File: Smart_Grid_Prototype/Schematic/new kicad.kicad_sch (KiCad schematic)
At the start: 78 parts, among them J1 EXT_POW, J2 AC_LOAD, J3 AC_STEPDOWN, J4 DC_LOAD, J5 POW_SHARE, J6 USB_C_Receptacle_PowerOnly_6P, J7 220VAC, J8 220VAC-TRANS, K1 G3MB-202PDC5, Q1 BD139, Q2 BD139, Q3 BD139, Q4 BD139, Q5 BD139, Q6 BD139, Q7 BD139, Q8 BD139, U1 ESP8266, U10 PC817, U11 PC817, U12 PC817, U13 PC817, U14 PC817, U15 PC817, U16 PC817, U2 RELAY_INT, U3 RELAY_PS, U4 PC817, U5 LM7824_TO220, U6 PC817, U7 PC817, U8 LM317_TO-220, U9 PC817

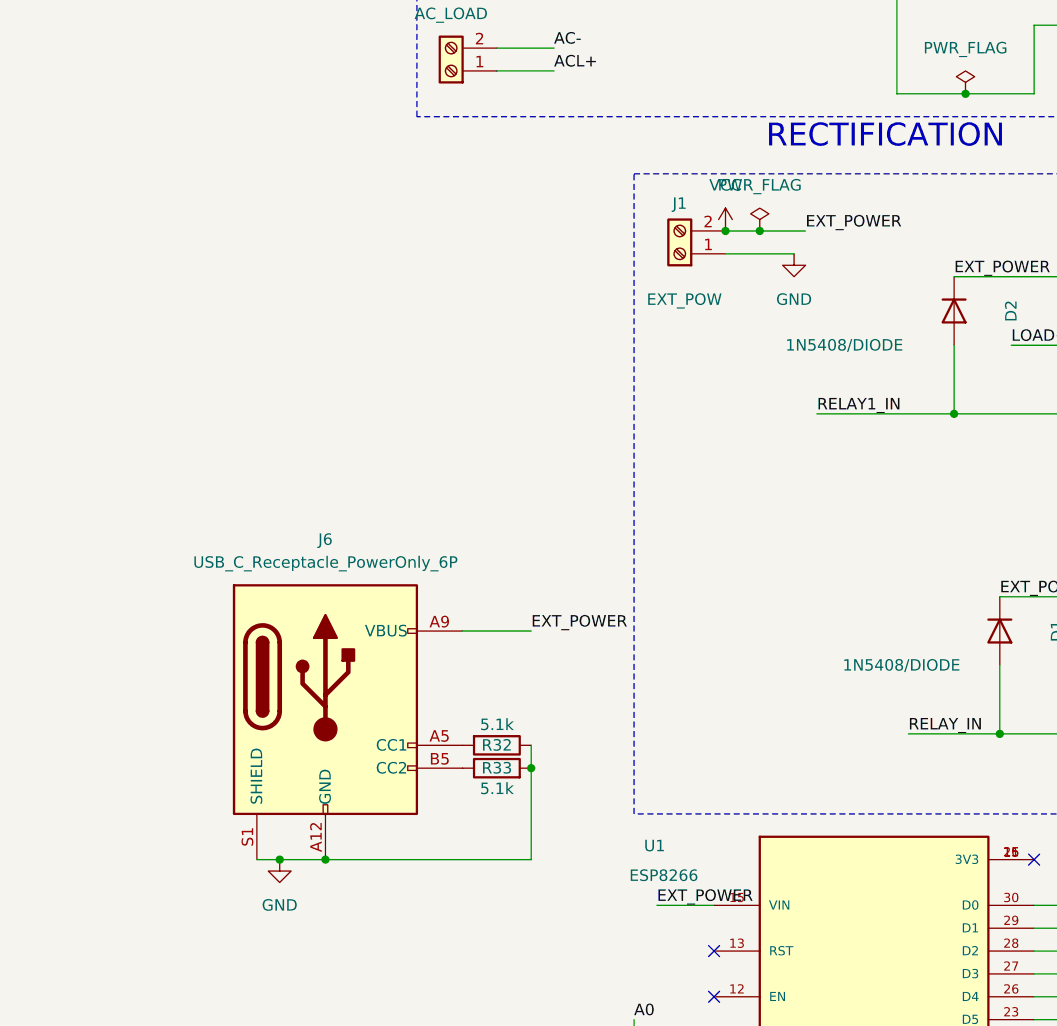
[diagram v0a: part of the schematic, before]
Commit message: finalised
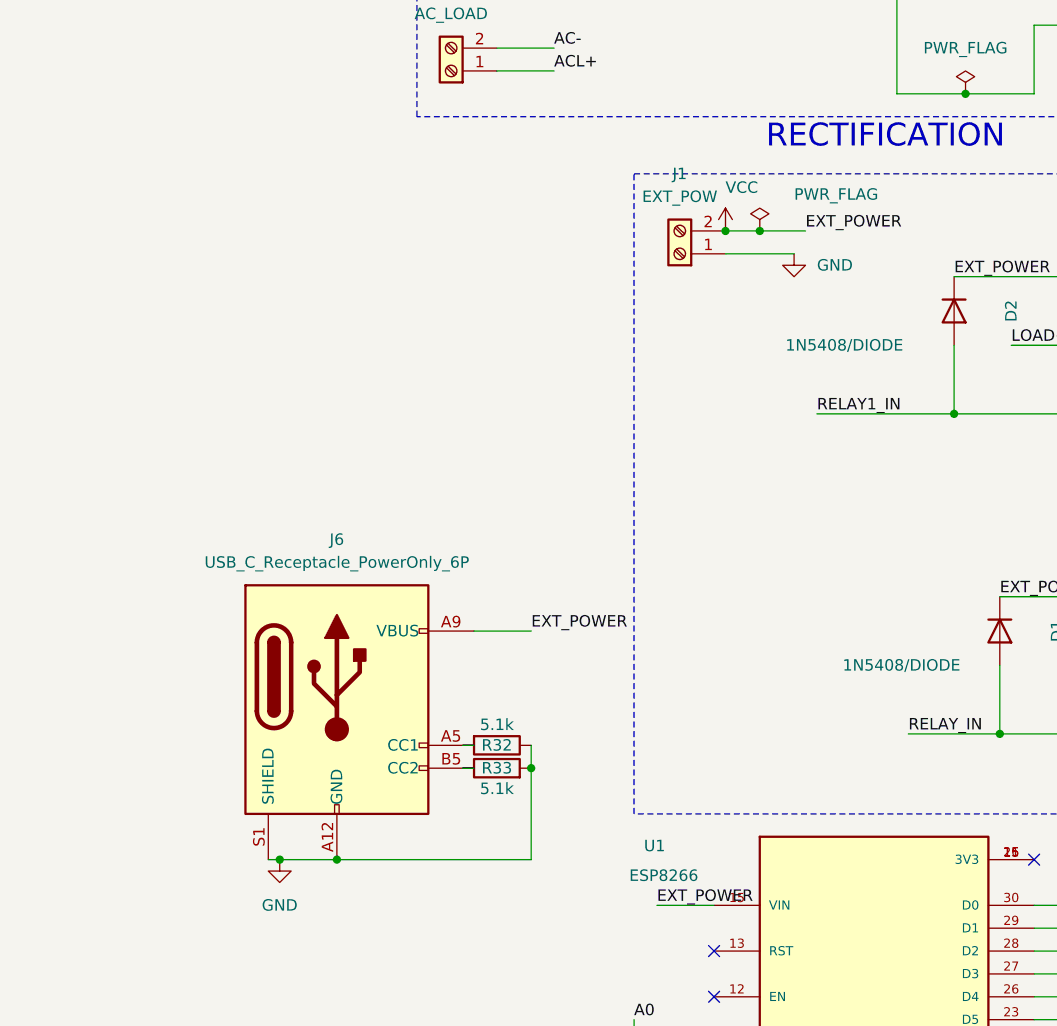
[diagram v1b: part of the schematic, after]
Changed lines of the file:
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@@
 	)
 	(junction
+		(at 69.85 166.37)
+		(diameter 0)
+		(color 0 0 0 0)
+	)
+	(junction
 		(at 139.7 81.28)
 		(diameter 0)
@@
 	)
 	(junction
-		(at 68.58 166.37)
-		(diameter 0)
-		(color 0 0 0 0)
-	)
-	(junction
 		(at 328.93 76.2)
 		(diameter 0)
@@
 	(wire
 		(pts
+			(xy 85.09 153.67) (xy 83.82 153.67)
+		)
+		(stroke
+			(width 0)
+			(type default)
+		)
+	)
+	(wire
+		(pts
 			(xy 323.85 68.58) (xy 323.85 77.47)
 		)
@@
 	(wire
 		(pts
+			(xy 85.09 156.21) (xy 83.82 156.21)
+		)
+		(stroke
+			(width 0)
+			(type default)
+		)
+	)
+	(wire
+		(pts
 			(xy 231.14 210.82) (xy 231.14 209.55)
 		)
@@
 	(wire
 		(pts
-			(xy 63.5 166.37) (xy 68.58 166.37)
-		)
-		(stroke
-			(width 0)
-			(type default)
-		)
-	)
-	(wire
-		(pts
 			(xy 294.64 72.39) (xy 284.48 72.39)
 		)
@@
 	(wire
 		(pts
+			(xy 69.85 166.37) (xy 91.44 166.37)
+		)
+		(stroke
+			(width 0)
+			(type default)
+		)
+	)
+	(wire
+		(pts
 			(xy 356.87 100.33) (xy 361.95 100.33)
 		)
@@
 	(wire
 		(pts
-			(xy 83.82 140.97) (xy 91.44 140.97)
+			(xy 85.09 140.97) (xy 91.44 140.97)
 		)
 		(stroke
@@
 	(wire
 		(pts
-			(xy 60.96 166.37) (xy 63.5 166.37)
+			(xy 62.23 166.37) (xy 63.5 166.37)
 		)
 		(stroke
@@
 	(wire
 		(pts
-			(xy 91.44 166.37) (xy 68.58 166.37)
+			(xy 63.5 166.37) (xy 69.85 166.37)
 		)
 		(stroke
@@
 		)
 		(property "Value" "GND"
-			(at 120.65 104.14 0)
+			(at 123.19 100.3299 0)
 			(effects
 				(font
 					(size 1.27 1.27)
 				)
+				(justify left)
 			)
 		)
@@
 		(on_board yes)
 		(dnp no)
-		(fields_autoplaced yes)
 		(property "Reference" "#PWR017"
 			(at 113.03 100.33 0)
@@
 		)
 		(property "Value" "VCC"
-			(at 113.03 91.44 0)
+			(at 113.03 91.694 0)
 			(effects
 				(font
 					(size 1.27 1.27)
 				)
+				(justify left)
 			)
 		)
@@
 		(on_board yes)
 		(dnp no)
-		(fields_autoplaced yes)
 		(property "Reference" "#FLG04"
 			(at 116.84 94.615 0)
@@
 		)
 		(property "Value" "PWR_FLAG"
-			(at 116.84 91.44 0)
+			(at 120.65 92.456 0)
 			(effects
 				(font
 					(size 1.27 1.27)
 				)
+				(justify left)
 			)
 		)
@@
 	)
 	(symbol
-		(lib_id "Connector:USB_C_Receptacle_PowerOnly_6P")
-		(at 68.58 148.59 0)
-		(unit 1)
-		(exclude_from_sim no)
-		(in_bom yes)
-		(on_board yes)
-		(dnp no)
-		(fields_autoplaced yes)
-		(property "Reference" "J6"
-			(at 68.58 130.81 0)
-			(effects
-				(font
-					(size 1.27 1.27)
-				)
-			)
-		)
-		(property "Value" "USB_C_Receptacle_PowerOnly_6P"
-			(at 68.58 133.35 0)
-			(effects
-				(font
-					(size 1.27 1.27)
-				)
-			)
-		)
-		(property "Footprint" "Connector_USB:USB_C_Receptacle_GCT_USB4125-xx-x-0190_6P_TopMnt_Horizontal"
-			(at 72.39 146.05 0)
-			(effects
-				(font
-					(size 1.27 1.27)
-				)
-				(hide yes)
-			)
-		)
-		(property "Datasheet" "https://www.usb.org/sites/default/files/documents/usb_type-c.zip"
-			(at 68.58 148.59 0)
-			(effects
-				(font
-					(size 1.27 1.27)
-				)
-				(hide yes)
-			)
-		)
-		(property "Description" "USB Power-Only 6P Type-C Receptacle connector"
-			(at 68.58 148.59 0)
-			(effects
-				(font
-					(size 1.27 1.27)
-				)
-				(hide yes)
-			)
-		)
-		(pin "S1"
-		)
-		(pin "B12"
-		)
-		(pin "B9"
-		)
-		(pin "B5"
-		)
-		(pin "A12"
-		)
-		(pin "A5"
-		)
-		(pin "A9"
-		)
-		(instances
-			(project ""
-				(path "/e03aa56c-38cd-4df1-a477-6f5e62efd874"
-					(reference "J6")
-					(unit 1)
-				)
-			)
-		)
-	)
-	(symbol
 		(lib_id "Device:R")
 		(at 53.34 49.53 270)
@@
 	)
 	(symbol
+		(lib_id "Connector:USB_C_Receptacle_PowerOnly_6P")
+		(at 69.85 148.59 0)
+		(unit 1)
+		(exclude_from_sim no)
+		(in_bom yes)
+		(on_board yes)
+		(dnp no)
+		(fields_autoplaced yes)
+		(property "Reference" "J6"
+			(at 69.85 130.81 0)
+			(effects
+				(font
+					(size 1.27 1.27)
+				)
+			)
+		)
+		(property "Value" "USB_C_Receptacle_PowerOnly_6P"
+			(at 69.85 133.35 0)
+			(effects
+				(font
+					(size 1.27 1.27)
+				)
+			)
+		)
+		(property "Footprint" "Connector_USB:USB_C_Receptacle_GCT_USB4125-xx-x-0190_6P_TopMnt_Horizontal"
+			(at 73.66 146.05 0)
+			(effects
+				(font
+					(size 1.27 1.27)
+				)
+				(hide yes)
+			)
+		)
+		(property "Datasheet" "https://www.usb.org/sites/default/files/documents/usb_type-c.zip"
+			(at 69.85 148.59 0)
+			(effects
+				(font
+					(size 1.27 1.27)
+				)
+				(hide yes)
+			)
+		)
+		(property "Description" "USB Power-Only 6P Type-C Receptacle connector"
+			(at 69.85 148.59 0)
+			(effects
+				(font
+					(size 1.27 1.27)
+				)
+				(hide yes)
+			)
+		)
+		(pin "B12"
+		)
+		(pin "B5"
+		)
+		(pin "A9"
+		)
+		(pin "A12"
+		)
+		(pin "B9"
+		)
+		(pin "S1"
+		)
+		(pin "A5"
+		)
+		(instances
+			(project ""
+				(path "/e03aa56c-38cd-4df1-a477-6f5e62efd874"
+					(reference "J6")
+					(unit 1)
+				)
+			)
+		)
+	)
+	(symbol
 		(lib_id "Device:R")
 		(at 168.91 57.15 0)
@@
 		(on_board yes)
 		(dnp no)
+		(fields_autoplaced yes)
 		(property "Reference" "J1"
-			(at 107.95 93.472 0)
+			(at 107.95 90.17 0)
 			(effects
 				(font
@@
 		)
 		(property "Value" "EXT_POW"
-			(at 108.458 104.14 0)
+			(at 107.95 92.71 0)
 			(effects
 				(font
